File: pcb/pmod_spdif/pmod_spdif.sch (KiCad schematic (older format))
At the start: 17 parts, among them J1 PMOD, J2 Conn_01x06_Male, U1 74HC04, U2 CAT3200-5, U3 TOTX1350(F), U4 SN74LVC1T45DBV

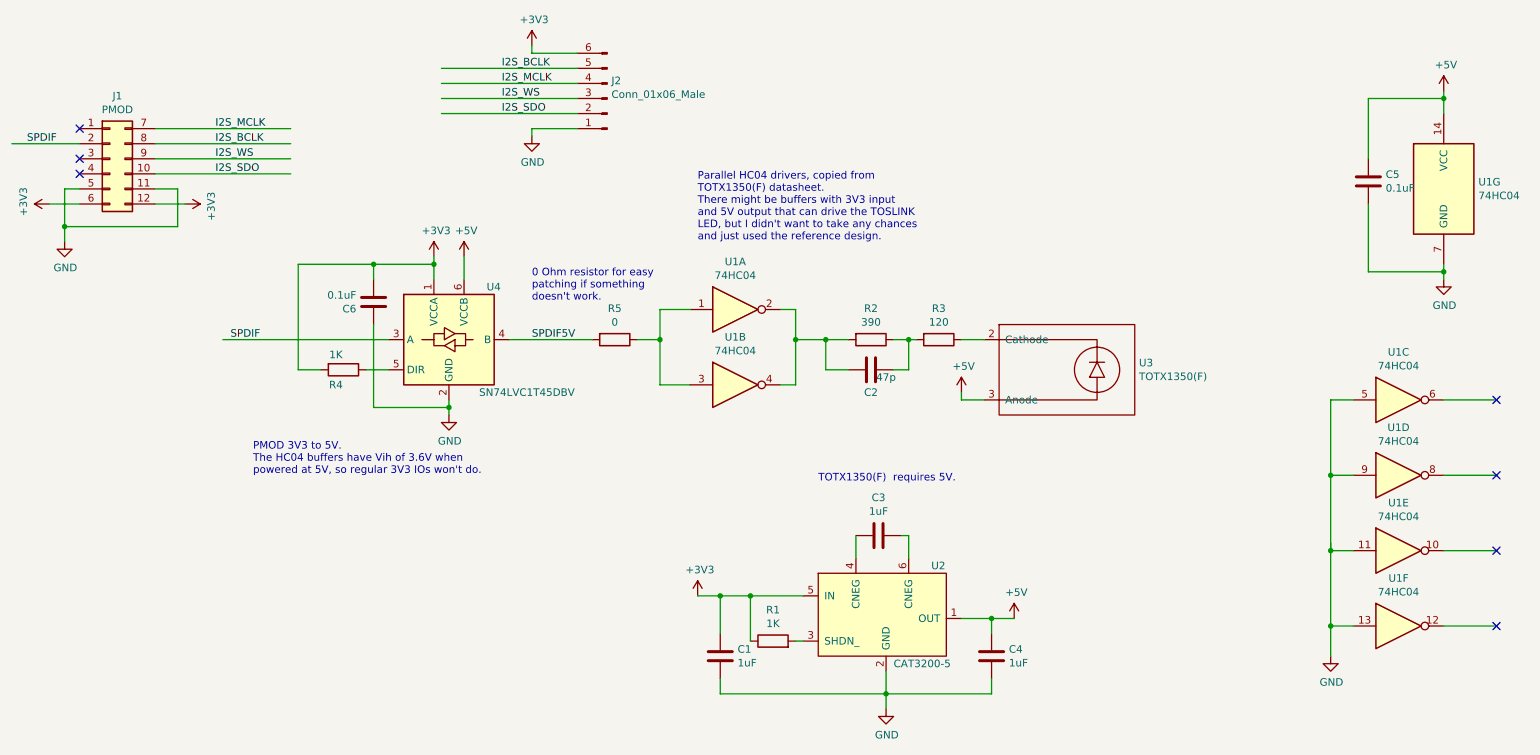
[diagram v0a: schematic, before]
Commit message: Update documentation.
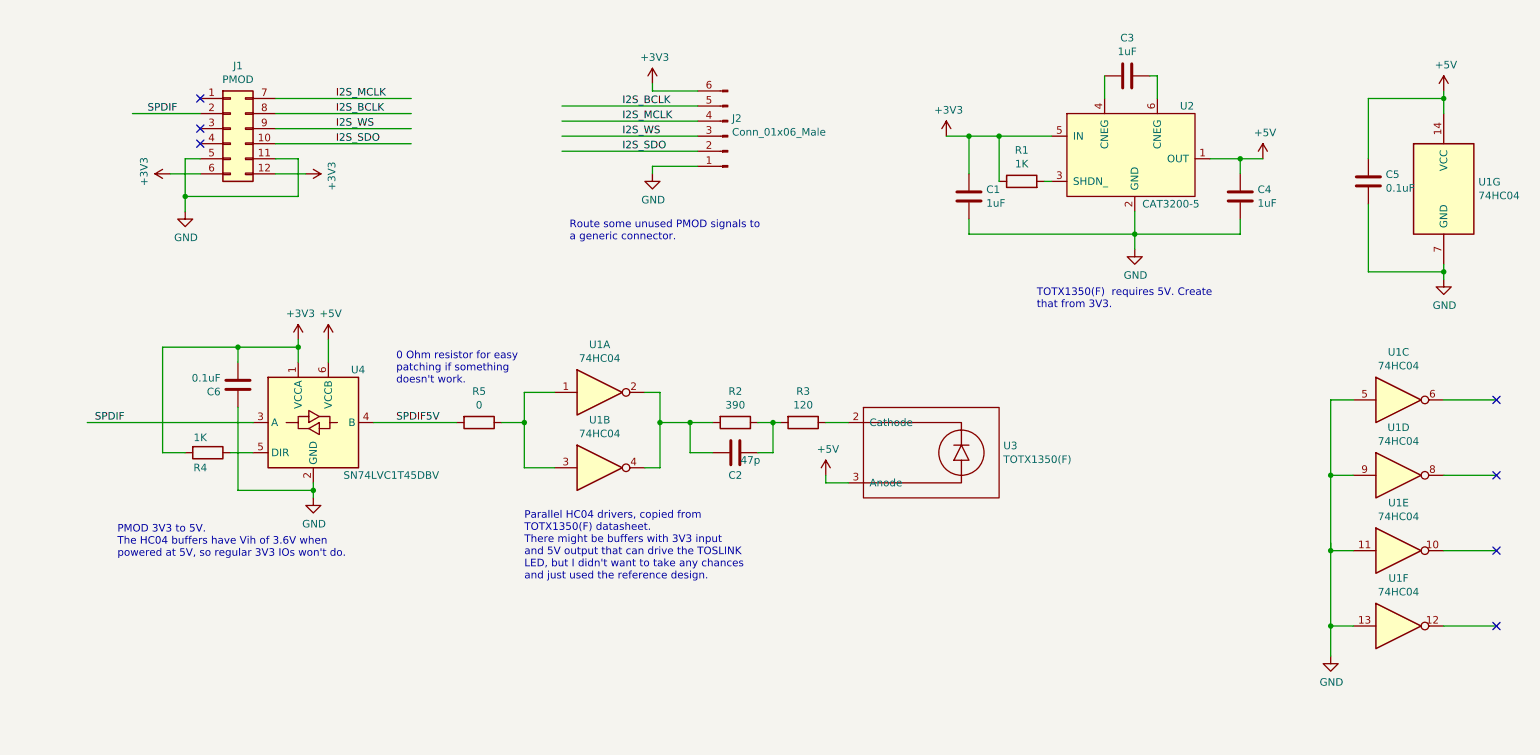
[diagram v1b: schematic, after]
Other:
- note added: "Route some unused PMOD signals to \na generic connector.\n"
- note added: "TOTX1350(F) requires 5V. Create\nthat from 3V3."
- note removed: "TOTX1350(F) requires 5V."
- moved on the sheet: C1, C2, C3, C4, C6, J1, J2, R1, R2, R3, R4, R5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
